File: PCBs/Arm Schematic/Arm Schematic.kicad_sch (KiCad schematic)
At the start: 89 parts, among them J1 USB_C_Receptacle_USB2.0_16P, J10 Conn_01x02, J11 Conn_01x04, J12 Conn_01x04, J13 Conn_01x02, J15 Conn_01x04, J16 Conn_01x05, J17 Conn_01x03, J2 Conn_01x05, J21 Conn_01x03, J22 Conn_01x03, J23 Conn_01x02, J24 Conn_01x04, J3 Conn_01x05, J4 Conn_01x05, J5 Conn_01x05, J6 Conn_01x04, J7 Conn_01x02, J8 Conn_01x02, J9 Conn_01x02, SW1 SW_Push, SW2 SW_Push, U1 ESP32-S3, U2 USBLC6-2SC6, U4 TCA9548APWR, U5 TXB0108DQSR, U6 TXB0108DQSR, U7 ADS1115IDGS, U8 W25Q16JVSS, U9 AMS1117-3.3, Y1 Crystal_GND24

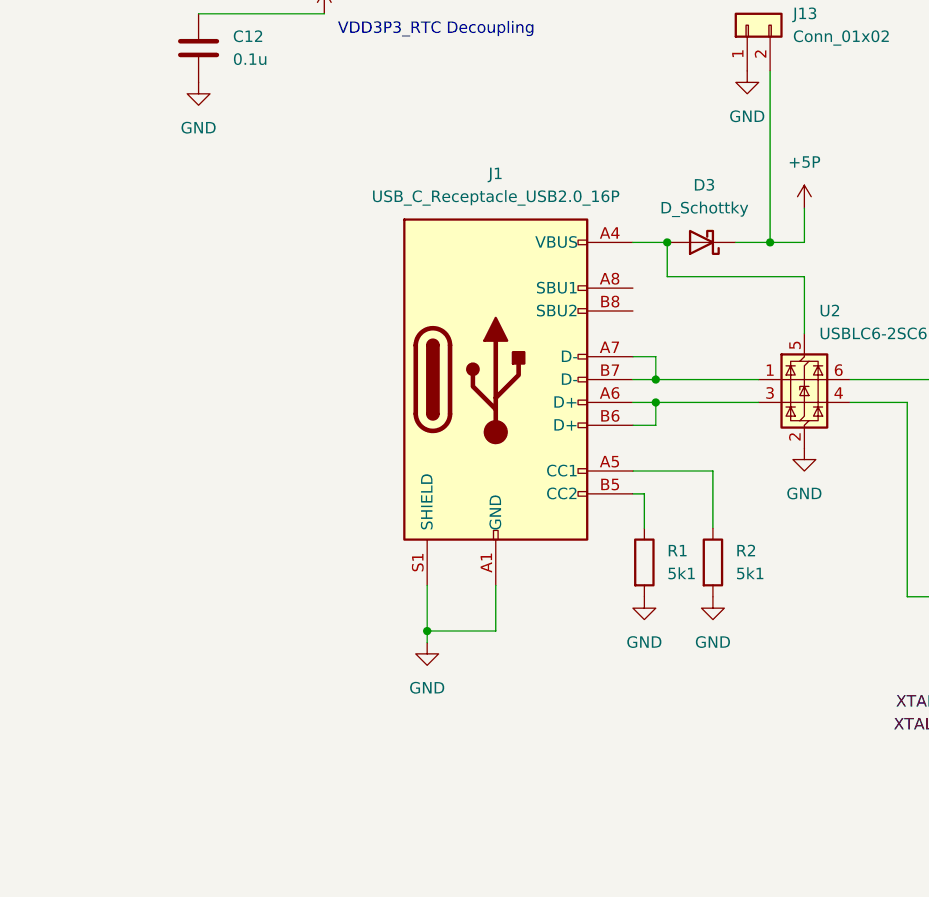
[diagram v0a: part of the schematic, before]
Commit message: Updated Arm PCB
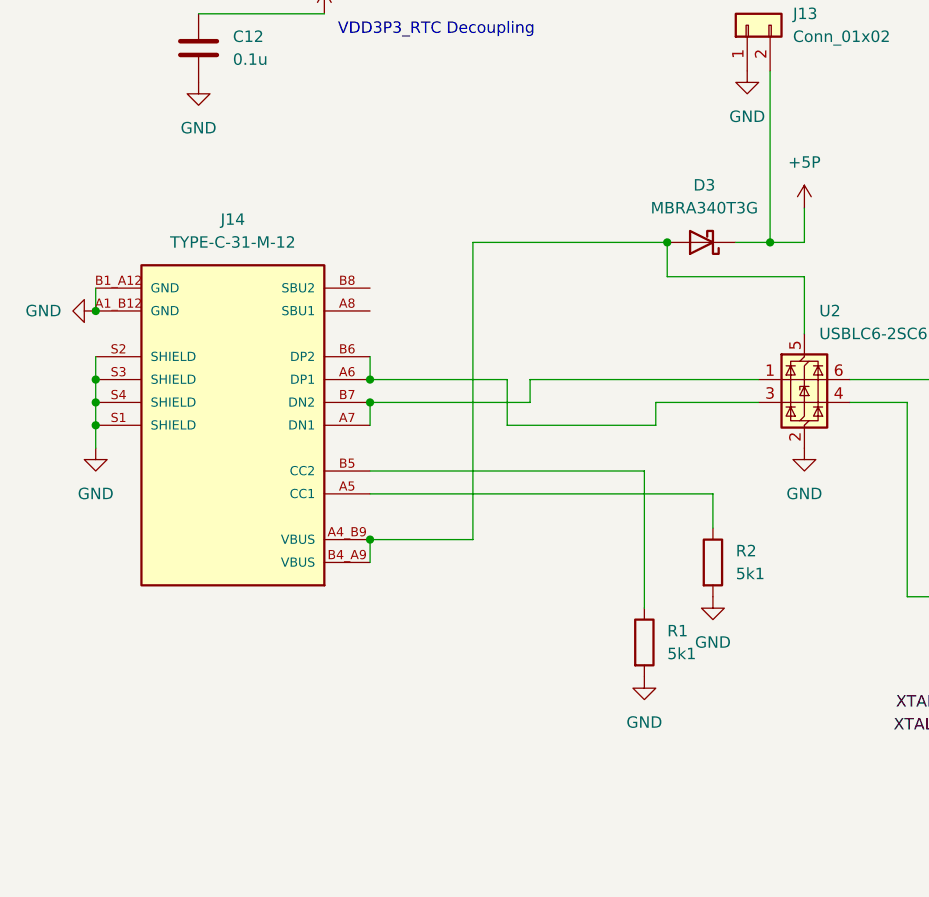
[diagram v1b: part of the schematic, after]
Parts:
- removed J1: USB_C_Receptacle_USB2.0_16P, Connector_USB:USB_C_Receptacle_GCT_USB4105-xx-A_16P_TopMnt_Horizontal, symbol Connector:USB_C_Receptacle_USB2.0_16P
- added J14: TYPE-C-31-M-12, IPRL Footprints:TYPE-C-31-M-12, symbol TYPE-C-31-M-12:TYPE-C-31-M-12
- D3: value D_Schottky -> MBRA340T3G; footprint Diode_SMD:D_0805_2012Metric -> Diode_SMD:D_SMA
- J13: footprint Connector_AMASS:AMASS_XT60-M_1x02_P7.20mm_Vertical -> Connector_AMASS:AMASS_XT30U-M_1x02_P5.0mm_Vertical
- Y1: footprint Oscillator:Oscillator_SMD_Abracon_ASDMB-4Pin_2.5x2.0mm -> Crystal:Crystal_SMD_SeikoEpson_FA238-4Pin_3.2x2.5mm
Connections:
- net GND: now also J14.A1_B12 (GND), J14.B1_A12 (GND), J14.S1 (SHIELD), J14.S2 (SHIELD), J14.S3 (SHIELD), J14.S4 (SHIELD)
- net at U2.1 (I/O1): now also J14.A7 (DN1), J14.B7 (DN2)
- net at U2.3 (I/O2): now also J14.A6 (DP1), J14.B6 (DP2)
- net at D3.2 (A), U2.5 (VBUS): now also J14.A4_B9 (VBUS), J14.B4_A9 (VBUS)
- net at R2.1: now also J14.A5 (CC1)
- net at R1.1: now also J14.B5 (CC2)
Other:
- moved on the sheet: R1
